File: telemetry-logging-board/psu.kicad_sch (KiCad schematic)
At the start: 30 parts, among them U10 AP61300Z6, U8 AP61300Z6, U9 AP61300Z6

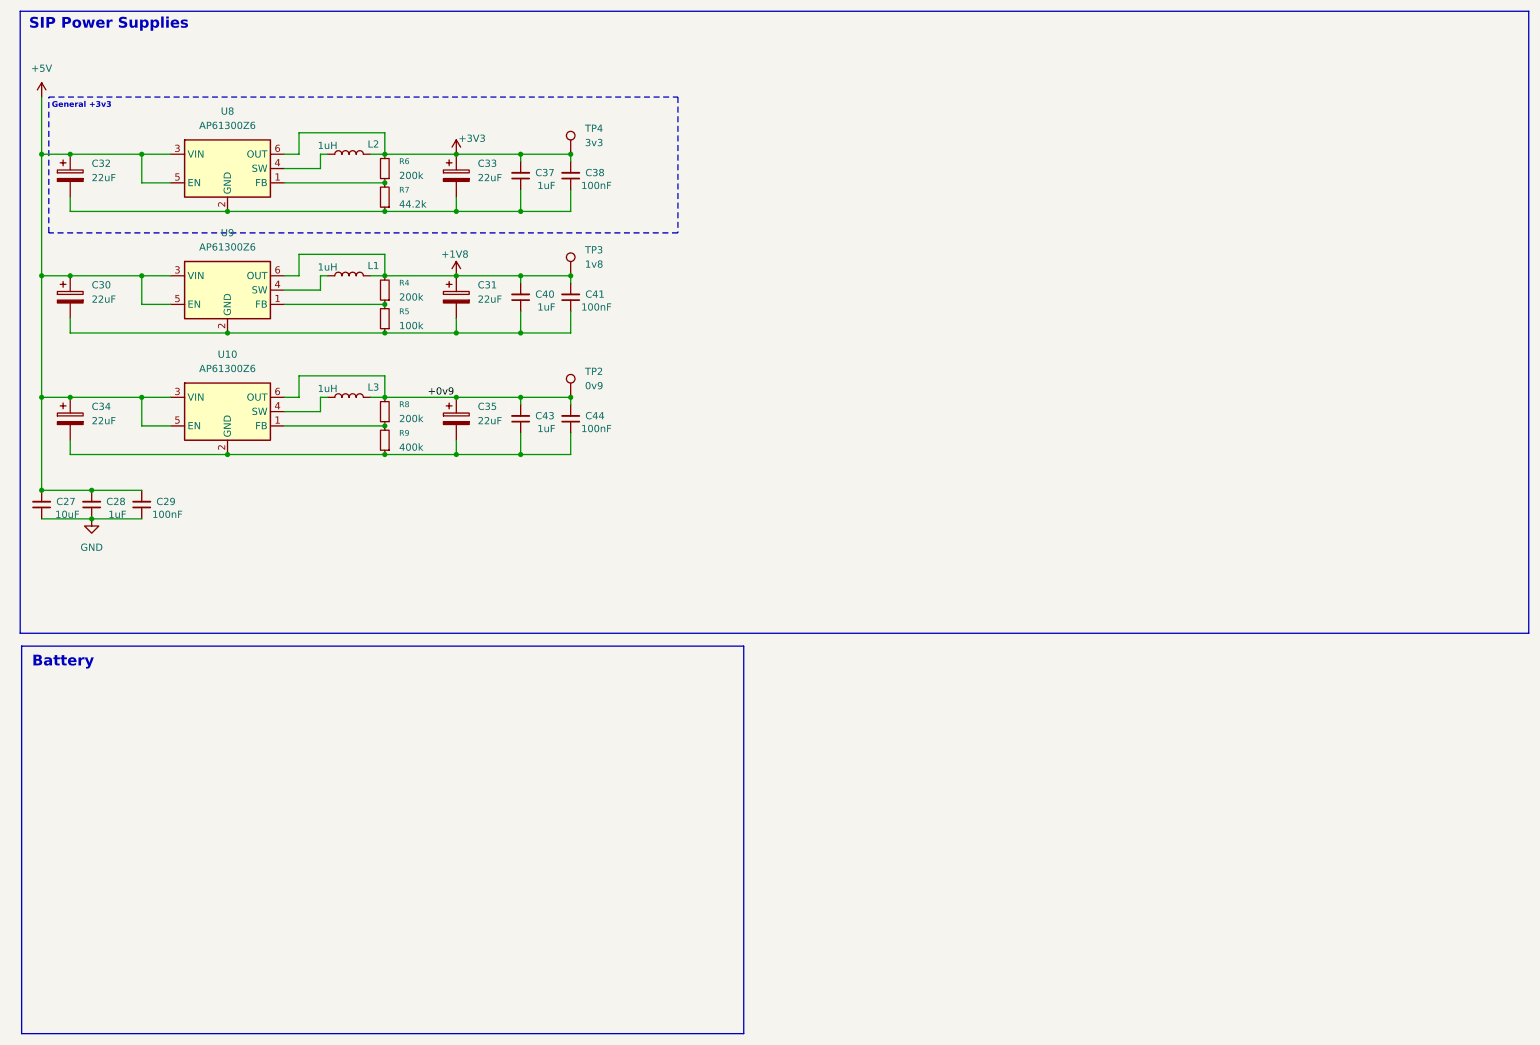
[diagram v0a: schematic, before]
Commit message: mostly CAN work
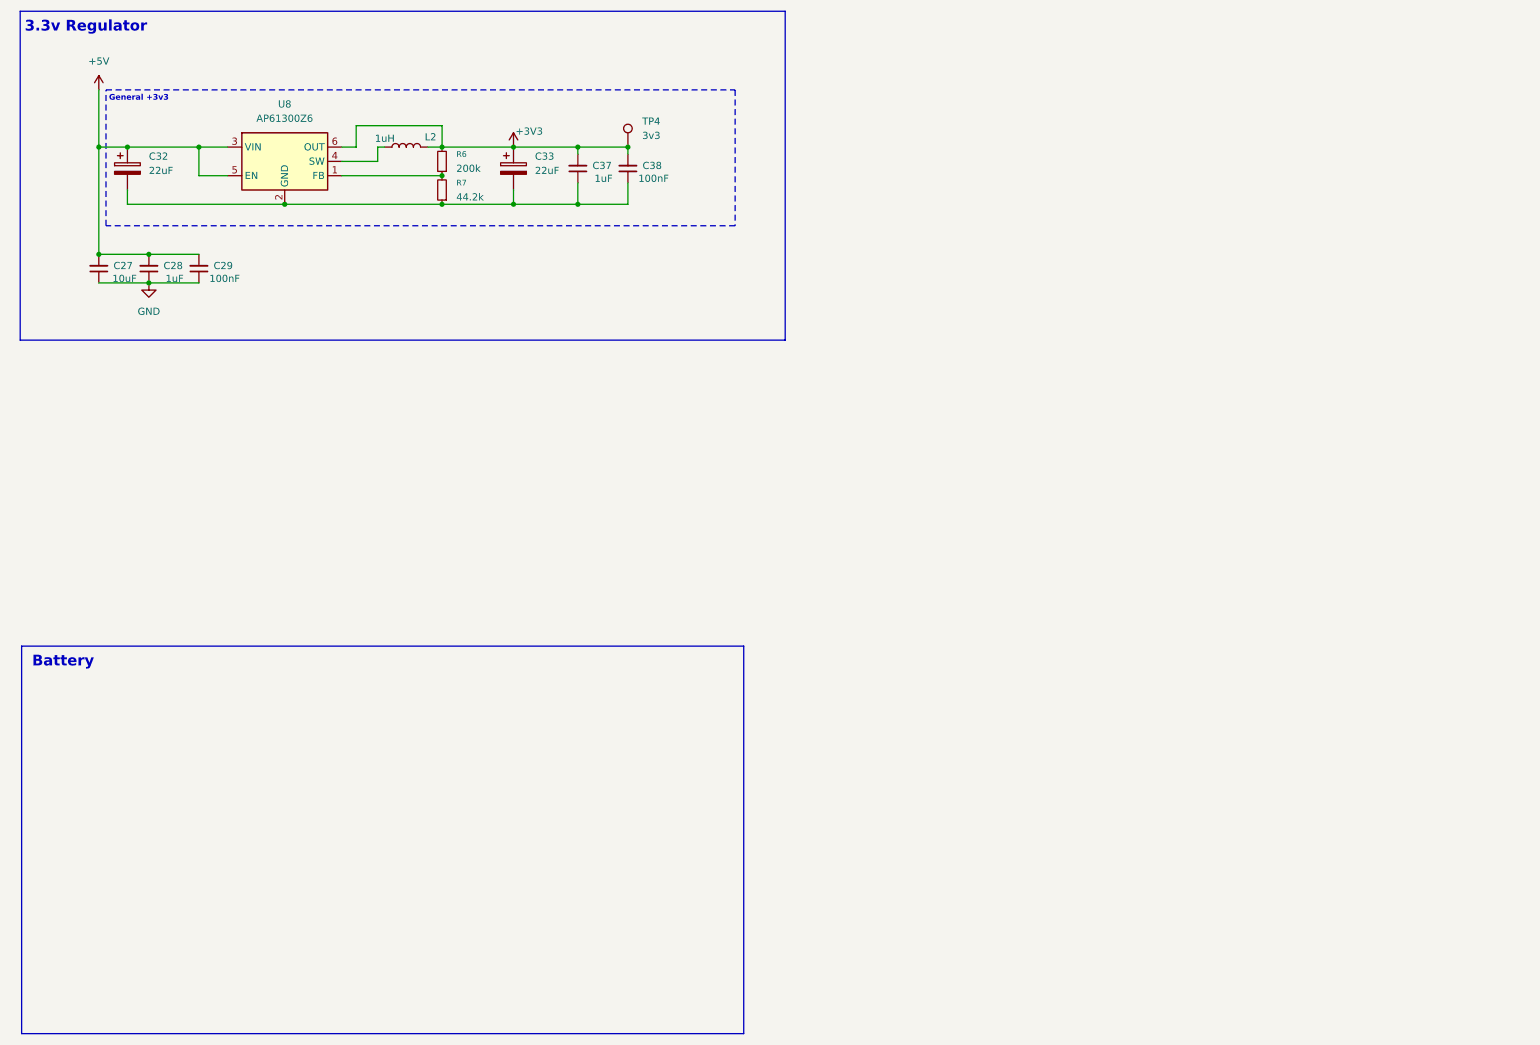
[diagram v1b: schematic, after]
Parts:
- removed C30, C31, C34, C35: 22uF, symbol Device:C_Polarized
- removed C40, C43: 1uF, symbol Device:C_Small
- removed C41, C44: 100nF, symbol Device:C_Small
- removed L1, L3: 1uH, symbol Device:L
- removed R4, R8: 200k, symbol Device:R_Small
- removed R5: 100k, symbol Device:R_Small
- removed R9: 400k, symbol Device:R_Small
- removed TP2: 0v9, symbol Connector:TestPoint
- removed TP3: 1v8, symbol Connector:TestPoint
- removed U10, U9: AP61300Z6, Package_TO_SOT_SMD:SOT-563, symbol Regulator_Switching:AP61300Z6
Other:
- note added: "3.3v Regulator"
- note removed: "SIP Power Supplies"
- company: (none) -> Formula Slug
- title: (none) -> Telemetry Logging Board
- moved on the sheet: C27, C28, C29, C32, C33, C37, C38, L2, R6, R7, TP4, U8
